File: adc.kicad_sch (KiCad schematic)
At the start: 8 parts, among them J1 Screw_Terminal_01x02, U1 Pico, U2 ADS8881CDGS, U3 LM4040DBZ-3

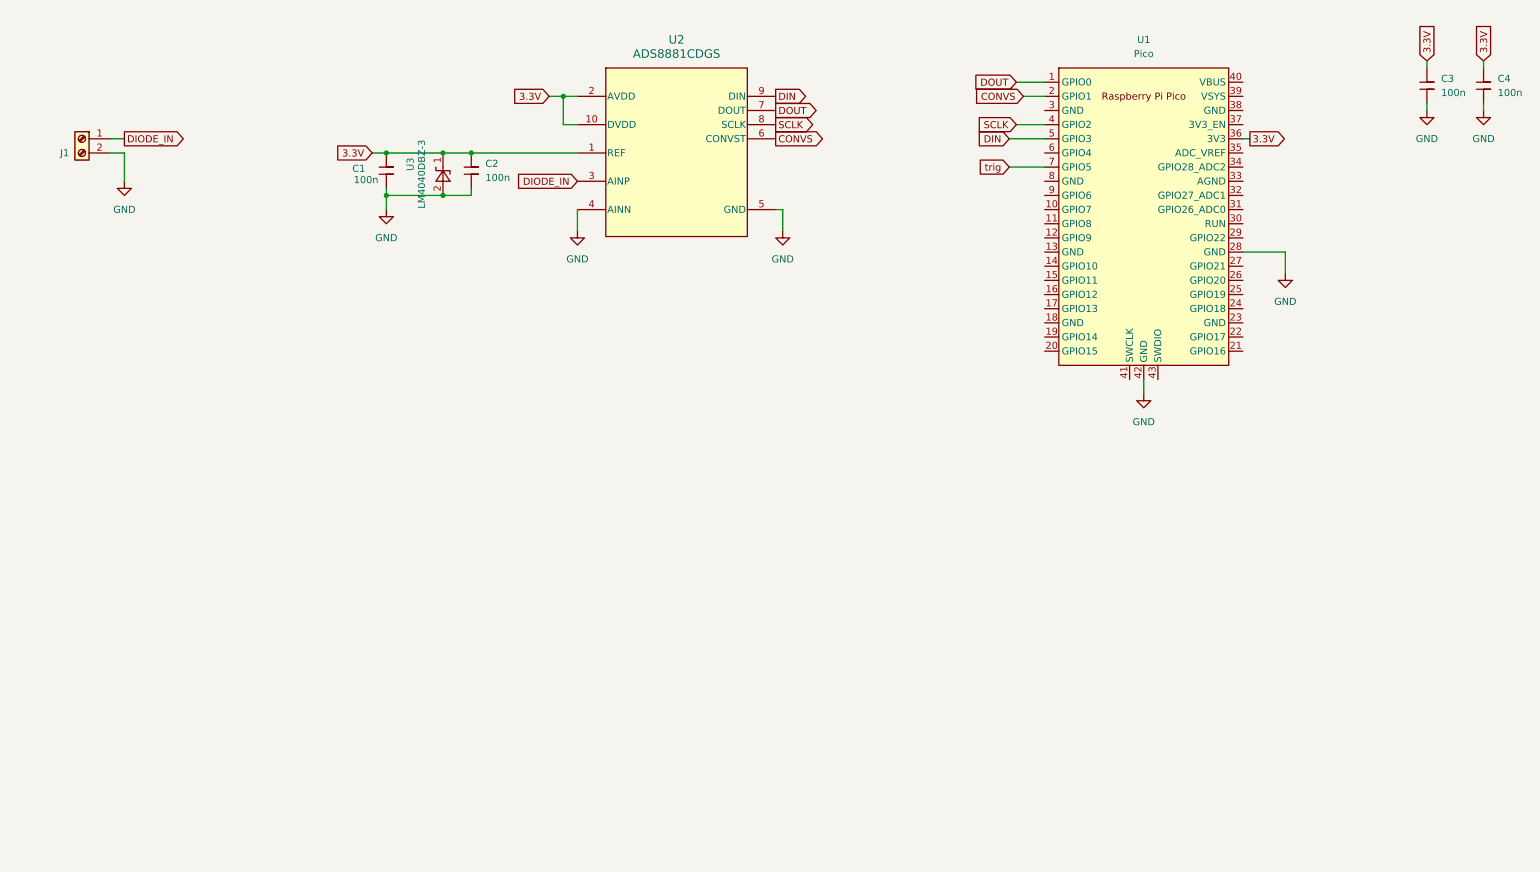
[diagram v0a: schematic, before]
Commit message: update 06.02.2025
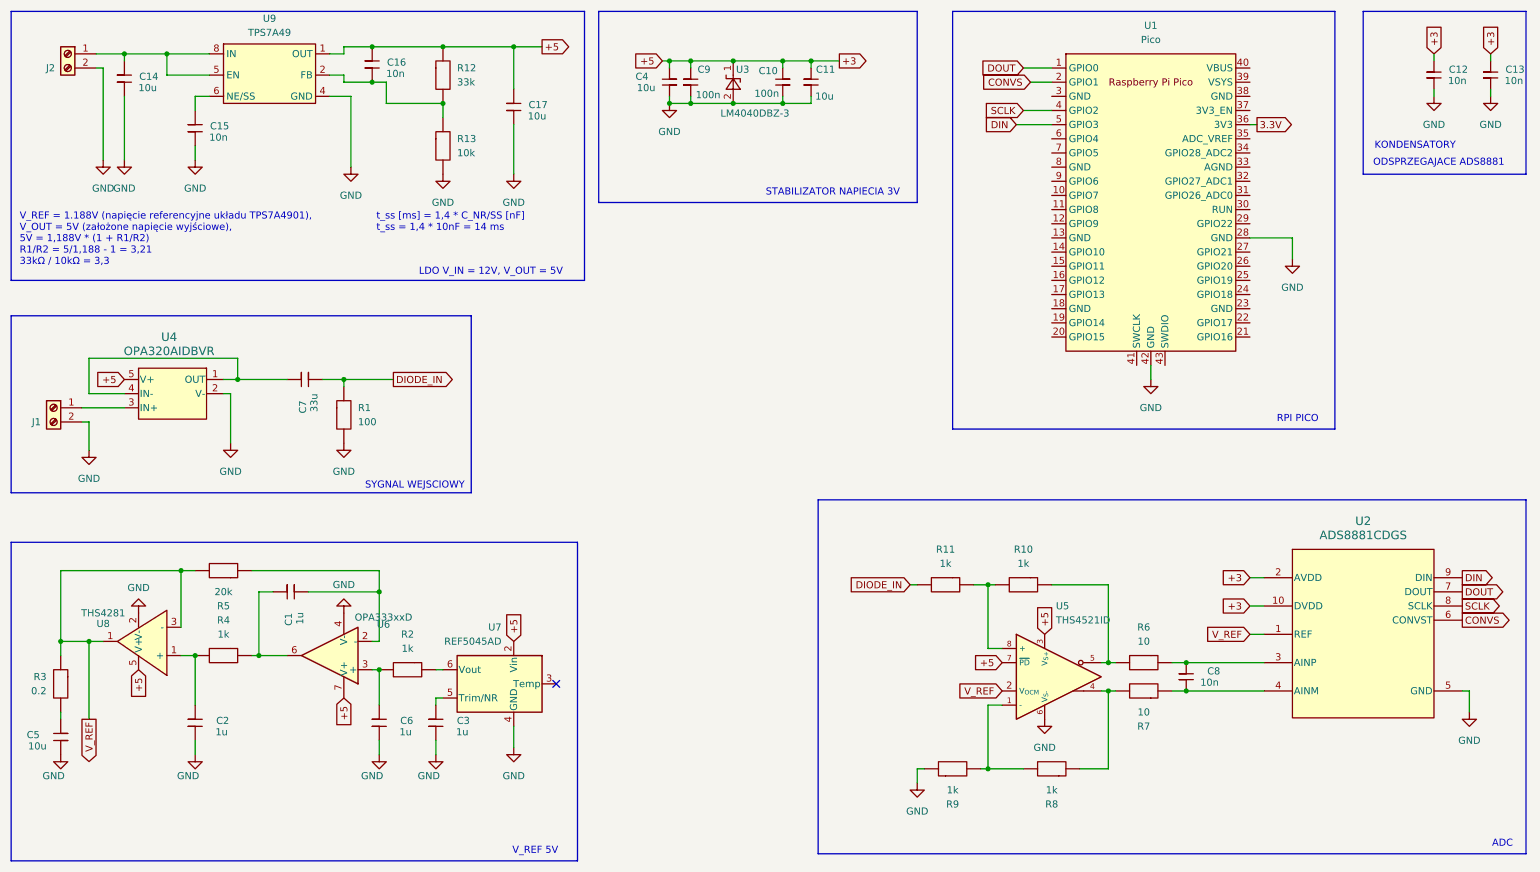
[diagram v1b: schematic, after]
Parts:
- added C10, C9: 100n, moja_biblioteka:cap_1206, symbol moja_biblioteka:cap_1206
- added C11, C14, C17, C5: 10u, moja_biblioteka:cap_1206, symbol moja_biblioteka:cap_1206
- added C12, C13, C15, C16, C8: 10n, moja_biblioteka:cap_1206, symbol moja_biblioteka:cap_1206
- added C6: 1u, moja_biblioteka:cap_1206, symbol moja_biblioteka:cap_1206
- added C7: 33u, moja_biblioteka:cap_1206, symbol moja_biblioteka:cap_1206
- added J2: Screw_Terminal_01x02, moja_biblioteka:screw_conector, symbol moja_biblioteka:Screw_Terminal_01x02
- added R1: 100, moja_biblioteka:res_1206, symbol moja_biblioteka:res_1206
- added R10, R11, R2, R4, R8, R9: 1k, moja_biblioteka:res_1206, symbol moja_biblioteka:res_1206
- added R12: 33k, moja_biblioteka:res_1206, symbol moja_biblioteka:res_1206
- added R13: 10k, moja_biblioteka:res_1206, symbol moja_biblioteka:res_1206
- added R3: 0.2, moja_biblioteka:res_1206, symbol moja_biblioteka:res_1206
- added R5: 20k, moja_biblioteka:res_1206, symbol moja_biblioteka:res_1206
- added R6, R7: 10, moja_biblioteka:res_1206, symbol moja_biblioteka:res_1206
- added U4: OPA320AIDBVR, OPA320:DBV5, symbol OPA320:OPA320AIDBVR
- added U5: THS4521ID, Package_SO:SOIC-8_3.9x4.9mm_P1.27mm, symbol Amplifier_Difference:THS4521ID
- added U6: OPA333xxD, Package_SO:SOIC-8_3.9x4.9mm_P1.27mm, symbol Amplifier_Operational:OPA333xxD
- added U7: REF5045AD, Package_SO:SOIC-8_3.9x4.9mm_P1.27mm, symbol Reference_Voltage:REF5045AD
- added U8: THS4281, moja_biblioteka:THS4281, symbol moja_biblioteka:THS4281
- added U9: TPS7A49, moja_biblioteka:THS4281, symbol moja_biblioteka:TPS7A49
- C1, C2, C3: value 100n -> 1u
- C4: value 100n -> 10u
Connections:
- net 3.3V: no longer C1.1, C2.1, C3.1, C4.1, U2.1 (REF), U2.10 (DVDD), U2.2 (AVDD), U3.1 (K)
- net DIODE_IN: now also C7.2, R1.1, R11.2; no longer J1.1 (Pin_1), U2.3 (AINP)
- net GND: now also C10.2, C11.2, C12.2, C13.2, C14.2, C15.2, C17.2, C5.2, C6.2, C9.2, J2.2 (Pin_2), R1.2, R13.2, R9.1, U4.2 (V-), U5.6 (V_{S-}), U6.4 (V-), U7.4 (GND), U8.2 (V-), U9.4 (GND); no longer C1.2, U2.4 (AINN)
- net trig: no longer names the net of U1.7 (GPIO5)
- new net: C3.1, U7.5 (Trim/NR)
- new net: R7.2, R8.1, U5.4
- new net: R8.2, R9.2, U5.1 (-)
- new net: C8.2, R7.1, U2.4 (AINM)
- new net: C15.1, U9.6 (NE/SS)
- new net: C16.2, R12.2, R13.1, U9.2 (FB)
- new net: C14.1, J2.1 (Pin_1), U9.5 (EN), U9.8 (IN)
- new net: C8.1, R6.1, U2.3 (AINP)
- new net: R10.1, R6.2, U5.5
- new net: C6.1, R2.2, U6.3 (+)
- new net: C7.1, U4.1 (OUT), U4.4 (IN-)
- new net: J1.1 (Pin_1), U4.3 (IN+)
- new net: C1.2, R5.1, U6.2 (-)
- new net: C1.1, R4.1, U6.6
- new net: R10.2, R11.1, U5.8 (+)
- new net: C5.1, R3.2
- new net: R2.1, U7.6 (Vout)
- new net: C2.1, R4.2, U8.1 (+)
- new net +3: C10.1, C11.1, C12.1, C13.1, C16.1, C17.1, C4.1, C9.1, R12.1, U2.10 (DVDD), U2.2 (AVDD), U3.1 (K), U4.5 (V+), U5.3 (V_{S+}), U5.7 (~{PD}), U6.7 (V+), U7.2 (Vin), U8.5 (V+), U9.1 (OUT)
- new net V_REF: R3.1, R5.2, U2.1 (REF), U5.2 (V_{OCM}), U8.1 (+), U8.3 (-)
- no-connect marks 0 -> 1
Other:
- note added: "5V = 1,188V * (1 + R1/R2) R1/R2 = 5/1,188 - 1 = 3,21 33kΩ / 10kΩ = 3,3"
- note added: "ADC"
- note added: "KONDENSATORY"
- note added: "LDO V_IN = 12V, V_OUT = 5V"
- note added: "ODSPRZEGAJACE ADS8881"
- note added: "RPI PICO"
- note added: "STABILIZATOR NAPIECIA 3V"
- note added: "SYGNAL WEJSCIOWY"
- note added: "V_REF 5V"
- note added: "V_REF = 1.188V (napięcie referencyjne układu TPS7A4901), V_OUT = 5V (założone napięcie wyjściowe),"
- note added: "t_ss [ms] = 1,4 * C_NR/SS [nF] t_ss = 1,4 * 10nF = 14 ms"
- moved on the sheet: J1, U1, U2
